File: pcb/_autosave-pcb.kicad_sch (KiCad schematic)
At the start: 136 parts, among them J1 Conn_02x20_JETSON, J10 Conn_01x02, J11 Conn_01x02, J12 Conn_01x02, J13 Conn_01x02, J14 Conn_01x02, J15 Conn_01x02, J16 Conn_01x02, J17 Conn_01x02, J18 Conn_01x04, J19 Conn_01x04, J2 Conn_02x22_STM32_LEFT, J2 Conn_02x22_STM32_RIGHT, J20 Conn_01x04, J21 Conn_01x04, J22 Conn_01x04, J23 Conn_01x04, J24 Conn_01x04, J25 Conn_01x04, J26 USB_B, J27 Conn_01x02, J28 Conn_02x22_Odd_Even_MountingP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, J29 Conn_02x22_Odd_Even_MountingP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, J3 Conn_24V, J31 Conn_ESC, J33 Conn_01x08, J4 Conn_ESC, J5 Conn_Servo, J6 Conn_01x02, J7 Conn_01x02, J8 Conn_01x02, J9 Conn_01x02, Q1 NPN, Q2 NPN, SW1 SW_DIP_x01, U1 PCA9685PW, U10 4001, U2 CP2102N-Axx-xQFN20, U3 74AHC244, U4 MCP6002-xMS, U5 MCP6002-xMS, U6 MCP6002-xMS, U7 MCP6002-xMS, U8 STM32F103C8Tx

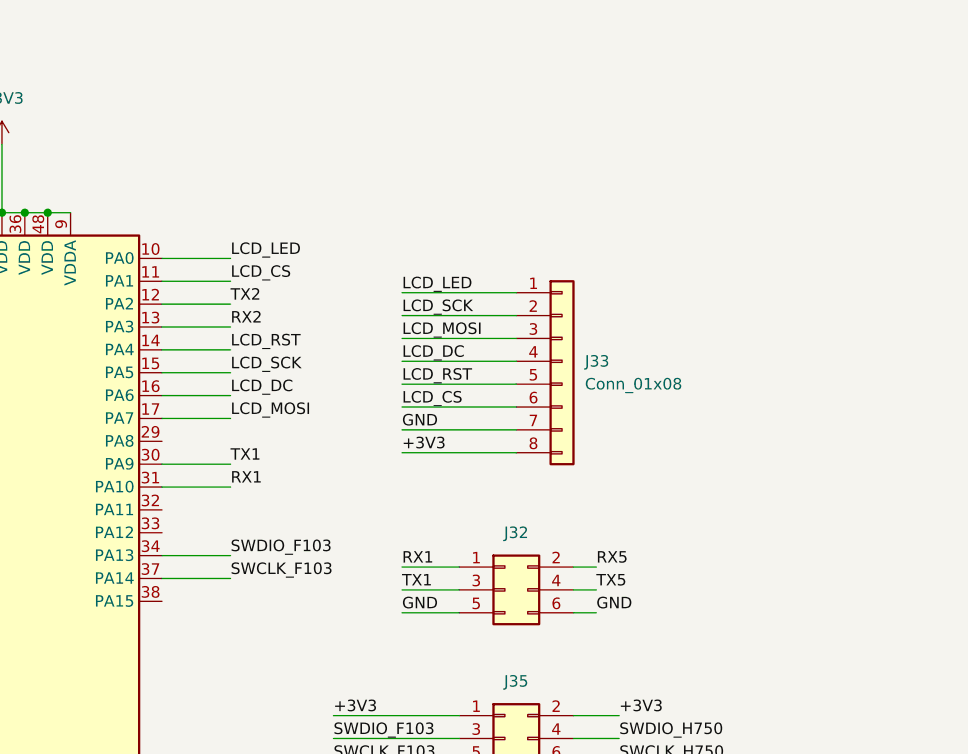
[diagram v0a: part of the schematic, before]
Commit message: first publish
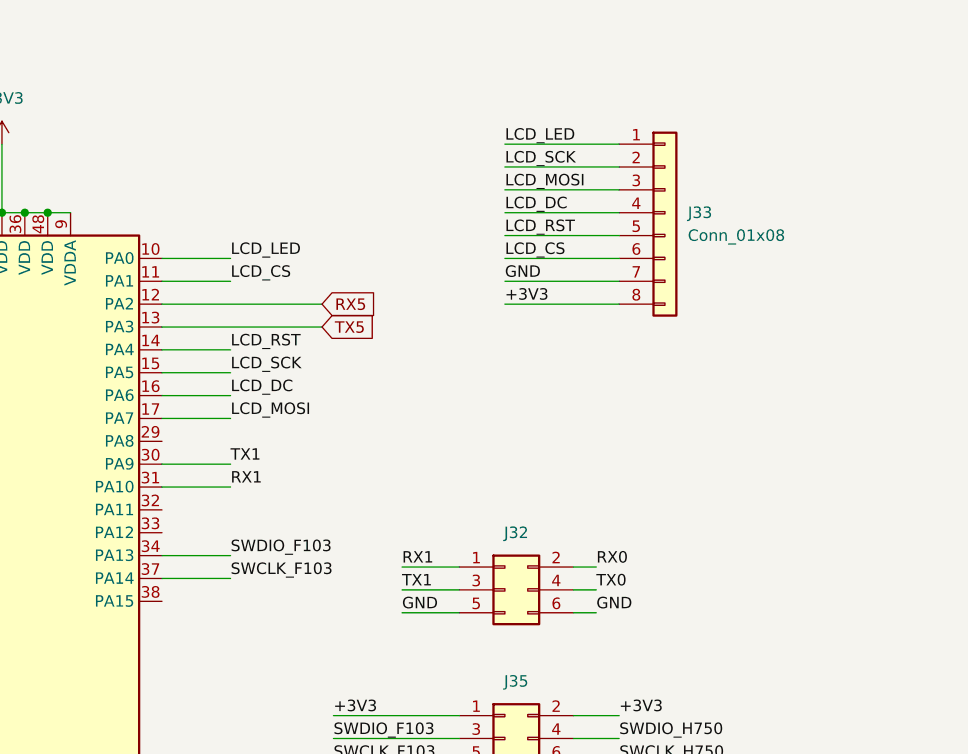
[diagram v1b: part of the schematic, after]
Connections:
- net RX2 is gone; now on net TX5: U8.13 (PA3)
- net TX2 is gone; now on net RX5: U8.12 (PA2)
- net RX0: now also J32.2 (Pin_2)
- net RX5: no longer J32.2 (Pin_2)
- net TX0: now also J32.4 (Pin_4)
- net TX5: no longer J32.4 (Pin_4)
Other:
- moved on the sheet: J33
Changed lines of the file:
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@@
     (stroke (width 0) (type default))
   )
-  (wire (pts (xy 163.83 50.8) (xy 171.45 50.8))
+  (wire (pts (xy 163.83 50.8) (xy 181.61 50.8))
     (stroke (width 0) (type default))
   )
@@
     (stroke (width 0) (type default))
   )
-  (wire (pts (xy 163.83 48.26) (xy 171.45 48.26))
+  (wire (pts (xy 163.83 48.26) (xy 181.61 48.26))
     (stroke (width 0) (type default))
   )
@@
     (stroke (width 0) (type default))
   )
-  (wire (pts (xy 190.5 59.69) (xy 203.2 59.69))
+  (wire (pts (xy 201.93 43.18) (xy 214.63 43.18))
     (stroke (width 0) (type default))
   )
@@
     (stroke (width 0) (type default))
   )
-  (wire (pts (xy 190.5 49.53) (xy 203.2 49.53))
+  (wire (pts (xy 201.93 33.02) (xy 214.63 33.02))
     (stroke (width 0) (type default))
   )
@@
     (stroke (width 0) (type default))
   )
-  (wire (pts (xy 190.5 52.07) (xy 203.2 52.07))
+  (wire (pts (xy 201.93 35.56) (xy 214.63 35.56))
     (stroke (width 0) (type default))
   )
@@
     (stroke (width 0) (type default))
   )
-  (wire (pts (xy 190.5 62.23) (xy 203.2 62.23))
+  (wire (pts (xy 201.93 45.72) (xy 214.63 45.72))
     (stroke (width 0) (type default))
   )
@@
     (stroke (width 0) (type default))
   )
-  (wire (pts (xy 190.5 46.99) (xy 203.2 46.99))
+  (wire (pts (xy 201.93 30.48) (xy 214.63 30.48))
     (stroke (width 0) (type default))
   )
@@
     (stroke (width 0) (type default))
   )
-  (wire (pts (xy 190.5 57.15) (xy 203.2 57.15))
+  (wire (pts (xy 201.93 40.64) (xy 214.63 40.64))
     (stroke (width 0) (type default))
   )
@@
     (stroke (width 0) (type default))
   )
-  (wire (pts (xy 190.5 54.61) (xy 203.2 54.61))
+  (wire (pts (xy 201.93 38.1) (xy 214.63 38.1))
     (stroke (width 0) (type default))
   )
@@
     (stroke (width 0) (type default))
   )
-  (wire (pts (xy 190.5 64.77) (xy 203.2 64.77))
+  (wire (pts (xy 201.93 48.26) (xy 214.63 48.26))
     (stroke (width 0) (type default))
   )
@@
     (effects (font (size 1.27 1.27)) (justify left bottom))
   )
-  (label "LCD_MOSI" (at 190.5 52.07 0) (fields_autoplaced)
+  (label "LCD_MOSI" (at 201.93 35.56 0) (fields_autoplaced)
     (effects (font (size 1.27 1.27)) (justify left bottom))
   )
@@
     (effects (font (size 1.27 1.27)) (justify left bottom))
   )
-  (label "LCD_LED" (at 190.5 46.99 0) (fields_autoplaced)
+  (label "LCD_LED" (at 201.93 30.48 0) (fields_autoplaced)
     (effects (font (size 1.27 1.27)) (justify left bottom))
   )
-  (label "GND" (at 190.5 62.23 0) (fields_autoplaced)
+  (label "GND" (at 201.93 45.72 0) (fields_autoplaced)
     (effects (font (size 1.27 1.27)) (justify left bottom))
   )
@@
     (effects (font (size 1.27 1.27)) (justify left bottom))
   )
-  (label "TX2" (at 171.45 48.26 0) (fields_autoplaced)
-    (effects (font (size 1.27 1.27)) (justify left bottom))
-  )
   (label "PD10" (at 59.69 223.52 0) (fields_autoplaced)
     (effects (font (size 1.27 1.27)) (justify left bottom))
@@
     (effects (font (size 1.27 1.27)) (justify left bottom))
   )
-  (label "LCD_SCK" (at 190.5 49.53 0) (fields_autoplaced)
+  (label "LCD_SCK" (at 201.93 33.02 0) (fields_autoplaced)
     (effects (font (size 1.27 1.27)) (justify left bottom))
   )
@@
     (effects (font (size 1.27 1.27)) (justify left bottom))
   )
-  (label "LCD_DC" (at 190.5 54.61 0) (fields_autoplaced)
+  (label "LCD_DC" (at 201.93 38.1 0) (fields_autoplaced)
     (effects (font (size 1.27 1.27)) (justify left bottom))
   )
@@
     (effects (font (size 1.27 1.27)) (justify left bottom))
   )
-  (label "RX5" (at 212.09 77.47 0) (fields_autoplaced)
+  (label "RX0" (at 212.09 77.47 0) (fields_autoplaced)
     (effects (font (size 1.27 1.27)) (justify left bottom))
   )
@@
     (effects (font (size 1.27 1.27)) (justify left bottom))
   )
-  (label "LCD_CS" (at 190.5 59.69 0) (fields_autoplaced)
+  (label "LCD_CS" (at 201.93 43.18 0) (fields_autoplaced)
     (effects (font (size 1.27 1.27)) (justify left bottom))
   )
@@
     (effects (font (size 1.27 1.27)) (justify left bottom))
   )
-  (label "+3V3" (at 190.5 64.77 0) (fields_autoplaced)
+  (label "+3V3" (at 201.93 48.26 0) (fields_autoplaced)
     (effects (font (size 1.27 1.27)) (justify left bottom))
   )
-  (label "TX5" (at 212.09 80.01 0) (fields_autoplaced)
+  (label "TX0" (at 212.09 80.01 0) (fields_autoplaced)
     (effects (font (size 1.27 1.27)) (justify left bottom))
   )
@@
     (effects (font (size 1.27 1.27)) (justify left bottom))
   )
-  (label "LCD_RST" (at 190.5 57.15 0) (fields_autoplaced)
+  (label "LCD_RST" (at 201.93 40.64 0) (fields_autoplaced)
     (effects (font (size 1.27 1.27)) (justify left bottom))
   )
@@
     (effects (font (size 1.27 1.27)) (justify left bottom))
   )
-  (label "RX2" (at 171.45 50.8 0) (fields_autoplaced)
-    (effects (font (size 1.27 1.27)) (justify left bottom))
-  )
   (label "PC5" (at 123.19 208.28 0) (fields_autoplaced)
     (effects (font (size 1.27 1.27)) (justify left bottom))
@@
     )
   )
+  (global_label "RX5" (shape input) (at 181.61 48.26 0) (fields_autoplaced)
+    (effects (font (size 1.27 1.27)) (justify left))
+    (property "Intersheetrefs" "${INTERSHEET_REFS}" (at 188.2842 48.26 0)
+      (effects (font (size 1.27 1.27)) (justify left) hide)
+    )
+  )
   (global_label "PB4{slash}OE" (shape input) (at -109.22 148.59 0) (fields_autoplaced)
     (effects (font (size 1.27 1.27)) (justify left))
@@
     )
   )
+  (global_label "TX5" (shape input) (at 181.61 50.8 0) (fields_autoplaced)
+    (effects (font (size 1.27 1.27)) (justify left))
+    (property "Intersheetrefs" "${INTERSHEET_REFS}" (at 187.9818 50.8 0)
+      (effects (font (size 1.27 1.27)) (justify left) hide)
+    )
+  )
   (global_label "PCA{slash}SERVO" (shape input) (at 350.52 33.02 0) (fields_autoplaced)
     (effects (font (size 1.27 1.27)) (justify left))
@@
     )
   )
-  (symbol (lib_id "Connector_Generic:Conn_01x08") (at 208.28 54.61 0) (unit 1)
+  (symbol (lib_id "Connector_Generic:Conn_01x08") (at 219.71 38.1 0) (unit 1)
     (in_bom yes) (on_board yes) (dnp no) (fields_autoplaced)
-    (property "Reference" "J33" (at 210.82 54.61 0)
+    (property "Reference" "J33" (at 222.25 38.1 0)
       (effects (font (size 1.27 1.27)) (justify left))
     )
-    (property "Value" "Conn_01x08" (at 210.82 57.15 0)
+    (property "Value" "Conn_01x08" (at 222.25 40.64 0)
       (effects (font (size 1.27 1.27)) (justify left))
     )
-    (property "Footprint" "" (at 208.28 54.61 0)
+    (property "Footprint" "" (at 219.71 38.1 0)
       (effects (font (size 1.27 1.27)) hide)
     )
-    (property "Datasheet" "~" (at 208.28 54.61 0)
+    (property "Datasheet" "~" (at 219.71 38.1 0)
       (effects (font (size 1.27 1.27)) hide)
     )

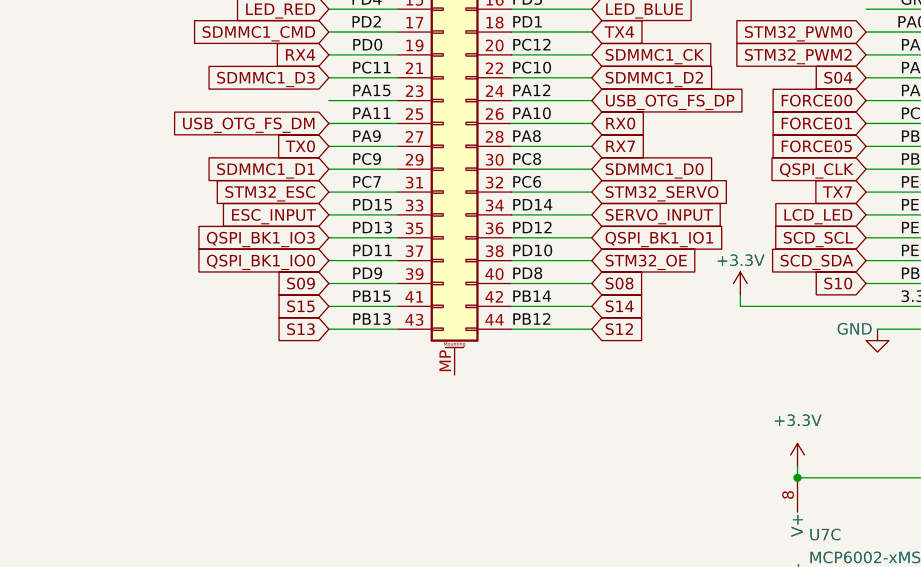
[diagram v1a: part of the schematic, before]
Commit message: first publish
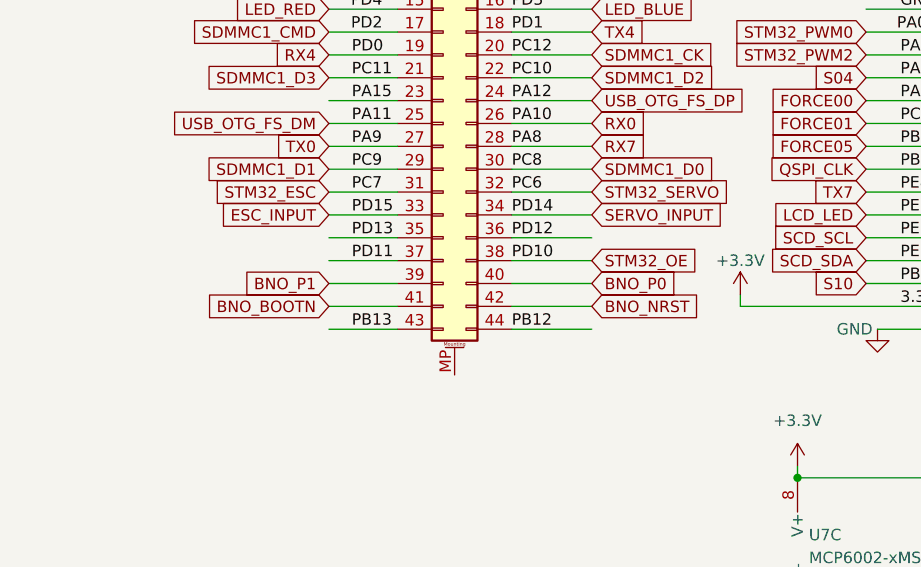
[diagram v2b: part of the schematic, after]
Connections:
- net S08: no longer J28.40 (Pin_40)
- net S09: no longer J28.39 (Pin_39)
- net S12: no longer J28.44 (Pin_44)
- net S13: no longer J28.43 (Pin_43)
- net S14: no longer J28.42 (Pin_42)
- net S15: no longer J28.41 (Pin_41)
- net QSPI_BK1_IO0 renamed PD11
- net QSPI_BK1_IO1 renamed PD12
- net QSPI_BK1_IO3 renamed PD13
- new net BNO_BOOTN: J28.41 (Pin_41)
- new net BNO_NRST: J28.42 (Pin_42)
- new net BNO_P0: J28.40 (Pin_40)
- new net BNO_P1: J28.39 (Pin_39)
- new net PB12: J28.44 (Pin_44)
- new net PB13: J28.43 (Pin_43)
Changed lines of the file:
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@@
-    (effects (font (size 1.27 1.27)) (justify left bottom))
-  )
-  (label "PD9" (at 41.91 226.06 0) (fields_autoplaced)
-    (effects (font (size 1.27 1.27)) (justify left bottom))
-  )
-  (label "PB14" (at 59.69 228.6 0) (fields_autoplaced)
     (effects (font (size 1.27 1.27)) (justify left bottom))
   )
@@
     (effects (font (size 1.27 1.27)) (justify left bottom))
   )
-  (label "PD8" (at 59.69 226.06 0) (fields_autoplaced)
-    (effects (font (size 1.27 1.27)) (justify left bottom))
-  )
   (label "PE12" (at 102.87 220.98 0) (fields_autoplaced)
     (effects (font (size 1.27 1.27)) (justify left bottom))
@@
     (effects (font (size 1.27 1.27)) (justify left bottom))
   )
-  (label "PB15" (at 41.91 228.6 0) (fields_autoplaced)
-    (effects (font (size 1.27 1.27)) (justify left bottom))
-  )
   (label "PE10" (at 102.87 218.44 0) (fields_autoplaced)
     (effects (font (size 1.27 1.27)) (justify left bottom))
@@
     )
   )
-  (global_label "QSPI_BK1_IO0" (shape input) (at 39.37 223.52 180) (fields_autoplaced)
-    (effects (font (size 1.27 1.27) (color 231 18 1 1)) (justify right))
-    (property "Intersheetrefs" "${INTERSHEET_REFS}" (at 23.1405 223.52 0)
-      (effects (font (size 1.27 1.27)) (justify right) hide)
-    )
-  )
   (global_label "PA7{slash}Force3" (shape input) (at -78.74 134.62 180) (fields_autoplaced)
     (effects (font (size 1.27 1.27)) (justify right))
@@
     (property "Intersheetrefs" "${INTERSHEET_REFS}" (at 147.4626 200.66 0)
       (effects (font (size 1.27 1.27)) (justify left) hide)
-    )
-  )
-  (global_label "S13" (shape input) (at 39.37 231.14 180) (fields_autoplaced)
-    (effects (font (size 1.27 1.27)) (justify right))
-    (property "Intersheetrefs" "${INTERSHEET_REFS}" (at 32.7563 231.14 0)
-      (effects (font (size 1.27 1.27)) (justify right) hide)
     )
   )
@@
     )
   )
+  (global_label "BNO_P1" (shape input) (at 39.37 226.06 180) (fields_autoplaced)
+    (effects (font (size 1.27 1.27)) (justify right))
+    (property "Intersheetrefs" "${INTERSHEET_REFS}" (at 29.0067 226.06 0)
+      (effects (font (size 1.27 1.27)) (justify right) hide)
+    )
+  )
   (global_label "PE6" (shape input) (at -53.34 149.86 0) (fields_autoplaced)
     (effects (font (size 1.27 1.27)) (justify left))
@@
     )
   )
-  (global_label "S14" (shape input) (at 68.58 228.6 0) (fields_autoplaced)
-    (effects (font (size 1.27 1.27)) (justify left))
-    (property "Intersheetrefs" "${INTERSHEET_REFS}" (at 75.1937 228.6 0)
-      (effects (font (size 1.27 1.27)) (justify left) hide)
-    )
-  )
   (global_label "vrs_6" (shape input) (at 86.36 387.35 180) (fields_autoplaced)
     (effects (font (size 1.27 1.27)) (justify right))
@@
     )
   )
-  (global_label "QSPI_BK1_IO3" (shape input) (at 39.37 220.98 180) (fields_autoplaced)
-    (effects (font (size 1.27 1.27) (color 231 18 1 1)) (justify right))
-    (property "Intersheetrefs" "${INTERSHEET_REFS}" (at 23.1405 220.98 0)
-      (effects (font (size 1.27 1.27)) (justify right) hide)
-    )
-  )
   (global_label "RX7" (shape input) (at 537.21 287.02 180) (fields_autoplaced)
     (effects (font (size 1.27 1.27)) (justify right))
@@
     )
   )
+  (global_label "BNO_P0" (shape input) (at 68.58 226.06 0) (fields_autoplaced)
+    (effects (font (size 1.27 1.27)) (justify left))
+    (property "Intersheetrefs" "${INTERSHEET_REFS}" (at 78.9433 226.06 0)
+      (effects (font (size 1.27 1.27)) (justify left) hide)
+    )
+  )
   (global_label "FORCE04" (shape input) (at 132.08 208.28 0) (fields_autoplaced)
     (effects (font (size 1.27 1.27)) (justify left))
@@
     )
   )
+  (global_label "BNO_BOOTN" (shape input) (at 39.37 228.6 180) (fields_autoplaced)
+    (effects (font (size 1.27 1.27)) (justify right))
+    (property "Intersheetrefs" "${INTERSHEET_REFS}" (at 25.2571 228.6 0)
+      (effects (font (size 1.27 1.27)) (justify right) hide)
+    )
+  )
   (global_label "Manual_Output" (shape input) (at 39.37 187.96 180) (fields_autoplaced)
     (effects (font (size 1.27 1.27)) (justify right))
@@
     )
   )
-  (global_label "QSPI_BK1_IO1" (shape input) (at 68.58 220.98 0) (fields_autoplaced)
-    (effects (font (size 1.27 1.27) (color 231 18 1 1)) (justify left))
-    (property "Intersheetrefs" "${INTERSHEET_REFS}" (at 84.8095 220.98 0)
-      (effects (font (size 1.27 1.27)) (justify left) hide)
-    )
-  )
   (global_label "S11" (shape input) (at 132.08 226.06 0) (fields_autoplaced)
     (effects (font (size 1.27 1.27)) (justify left))
@@
     )
   )
-  (global_label "S09" (shape input) (at 39.37 226.06 180) (fields_autoplaced)
-    (effects (font (size 1.27 1.27)) (justify right))
-    (property "Intersheetrefs" "${INTERSHEET_REFS}" (at 32.7563 226.06 0)
-      (effects (font (size 1.27 1.27)) (justify right) hide)
-    )
-  )
   (global_label "TX5" (shape input) (at 181.61 50.8 0) (fields_autoplaced)
     (effects (font (size 1.27 1.27)) (justify left))
@@
     (property "Intersheetrefs" "${INTERSHEET_REFS}" (at 127.5057 349.25 0)
       (effects (font (size 1.27 1.27)) (justify left) hide)
-    )
-  )
-  (global_label "S15" (shape input) (at 39.37 228.6 180) (fields_autoplaced)
-    (effects (font (size 1.27 1.27)) (justify right))
-    (property "Intersheetrefs" "${INTERSHEET_REFS}" (at 32.7563 228.6 0)
-      (effects (font (size 1.27 1.27)) (justify right) hide)
     )
   )
@@
     )
   )
-  (global_label "S12" (shape input) (at 68.58 231.14 0) (fields_autoplaced)
-    (effects (font (size 1.27 1.27)) (justify left))
-    (property "Intersheetrefs" "${INTERSHEET_REFS}" (at 75.1937 231.14 0)
-      (effects (font (size 1.27 1.27)) (justify left) hide)
-    )
-  )
   (global_label "USB_OTG_FS_DP" (shape input) (at 68.58 205.74 0) (fields_autoplaced)
     (effects (font (size 1.27 1.27) (color 231 18 1 1)) (justify left))
@@
     )
   )
-  (global_label "S08" (shape input) (at 68.58 226.06 0) (fields_autoplaced)
-    (effects (font (size 1.27 1.27)) (justify left))
-    (property "Intersheetrefs" "${INTERSHEET_REFS}" (at 75.1937 226.06 0)
-      (effects (font (size 1.27 1.27)) (justify left) hide)
-    )
-  )
   (global_label "PB6{slash}SDA" (shape input) (at -110.49 151.13 0) (fields_autoplaced)
     (effects (font (size 1.27 1.27)) (justify left))
@@
     )
   )
+  (global_label "BNO_NRST" (shape input) (at 68.58 228.6 0) (fields_autoplaced)
+    (effects (font (size 1.27 1.27)) (justify left))
+    (property "Intersheetrefs" "${INTERSHEET_REFS}" (at 81.2414 228.6 0)
+      (effects (font (size 1.27 1.27)) (justify left) hide)
+    )
+  )
